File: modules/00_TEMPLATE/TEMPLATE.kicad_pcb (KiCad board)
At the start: 2 copper layers, 160 x 100 mm, 2 parts, among them J1 Card_Connector

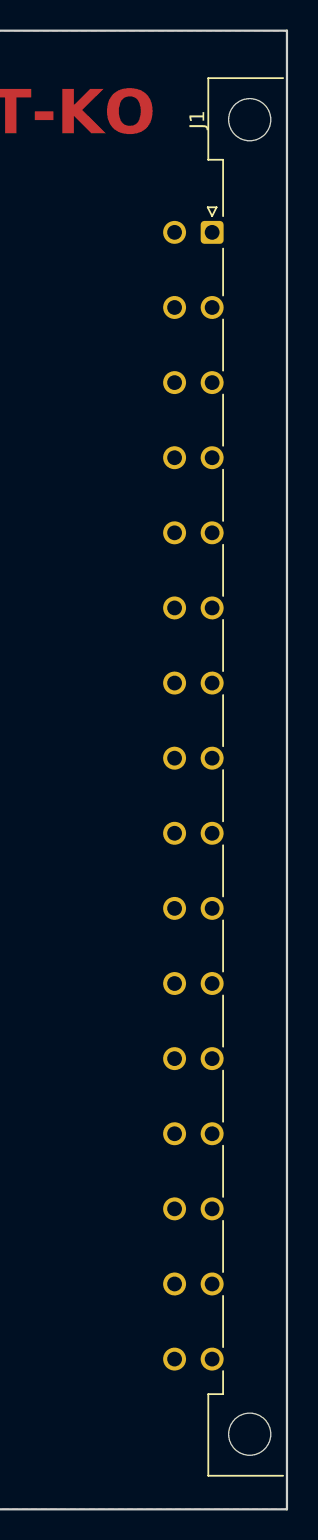
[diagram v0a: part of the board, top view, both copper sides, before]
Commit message: panel updates & vco
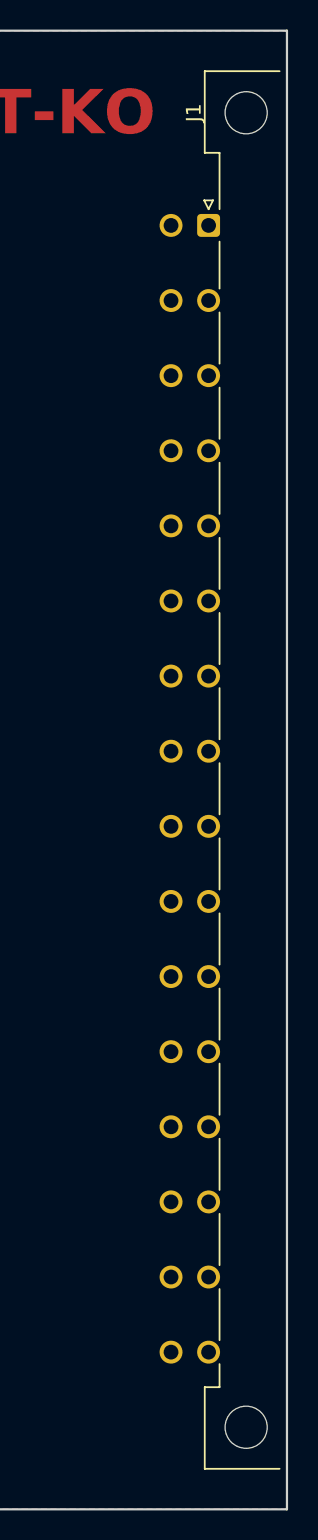
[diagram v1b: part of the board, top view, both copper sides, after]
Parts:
- moved J1 40.2 mm to (215.0, 95.0)
